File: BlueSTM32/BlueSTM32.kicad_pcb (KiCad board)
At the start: 4 copper layers, 40 x 40 mm, 63 parts, among them J1 TC2030-NL, J2 522071233, J3 USB4500-03-1-A_REVA, U1 OPA340NA, U2 BQ24040DSQR, U4 REF2033, U5 LT1304CS8-3.3-PBF, U6 LSM6DSRTR, U7 W25N02KVZEIR TR, U8 STM32WB55RGVx, X3 32.768kHz, X4 32MHz

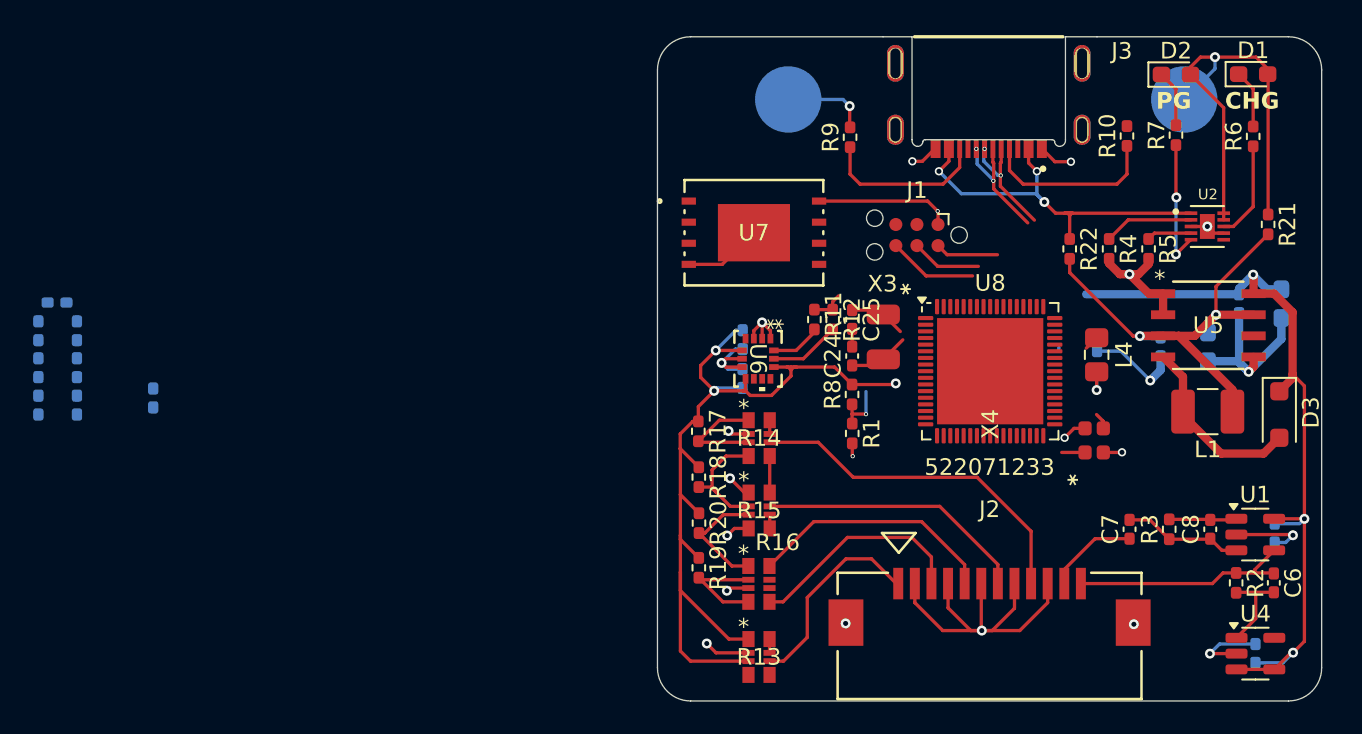
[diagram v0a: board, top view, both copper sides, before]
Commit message: Final layout of board
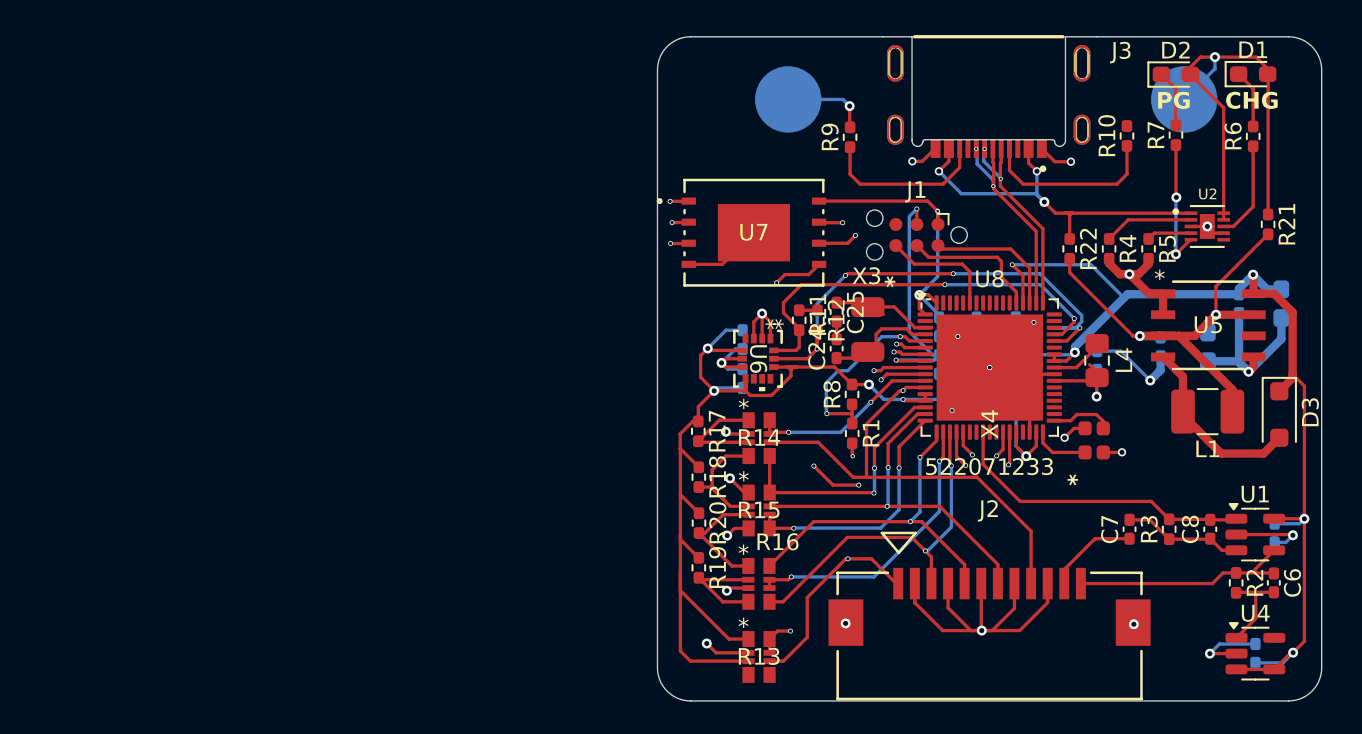
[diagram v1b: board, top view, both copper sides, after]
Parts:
- moved C18 58.9 mm to (171.6, 117.5), turned to 90 degrees
- moved C16 56.6 mm to (171.6, 119.7)
- moved C19 55.5 mm to (169.2, 119.7), turned to -90 degrees
- moved C20 54.4 mm to (167.0, 117.5)
- moved C21 54.4 mm to (169.2, 117.5), turned to -90 degrees
- moved C17 54.3 mm to (169.2, 122.0), turned to -90 degrees
- moved C1 54.2 mm to (167.0, 119.7), turned to -90 degrees
- moved C22 52.0 mm to (171.6, 122.0), turned to 90 degrees
- moved C25 1.03 mm to (160.8, 116.6)
- moved C24 1.03 mm to (160.8, 118.8)
- moved X3 1.03 mm to (162.7, 116.3)
- moved R12 0.92 mm to (159.6, 117.1)
- moved R11 0.92 mm to (158.5, 117.1)
- moved L4 0.35 mm to (176.5, 119.5)
- moved U8 0.22 mm to (170.0, 119.9)
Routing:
- net +3V3: track 116.4 -> 170.8 mm, vias 7 -> 12
- net /Microcontroller/Flash_CS: track 0.00 -> 35.5 mm, vias 0 -> 2
- net /Microcontroller/Flash_WP(IO2): track 0.00 -> 31.7 mm, vias 0 -> 4
- net IMU_SCL: track 4.27 -> 30.5 mm, vias 0 -> 4
- net Thermistor_Sense_+: track 0.83 -> 23.4 mm, vias 0 -> 2
- net IMU_SDA: track 3.06 -> 25.3 mm, vias 0 -> 2
- net /Microcontroller/Flash_CLK: track 0.00 -> 22.1 mm, vias 0 -> 2
- net /Microcontroller/Flash_HOLD(IO3): track 0.00 -> 21.4 mm, vias 0 -> 2
- net GND: track 94.1 -> 114.0 mm, vias 22 -> 27
- net /Microcontroller/Flash_DO(IO1): track 0.00 -> 19.4 mm, vias 0 -> 2
- net Strain_4_Sense_+: track 0.00 -> 17.3 mm, vias 0 -> 2
- net /Microcontroller/SWD_RST: track 0.00 -> 15.4 mm, vias 0 -> 2
- net Thermistor_Sense_-: track 12.3 -> 27.4 mm, vias 0 -> 2
- net Piezoelectric_Out: track 4.08 -> 18.6 mm
- net Strain_3_Sense_+: track 0.83 -> 15.1 mm, vias 0 -> 2
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
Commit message: Better Final Layout
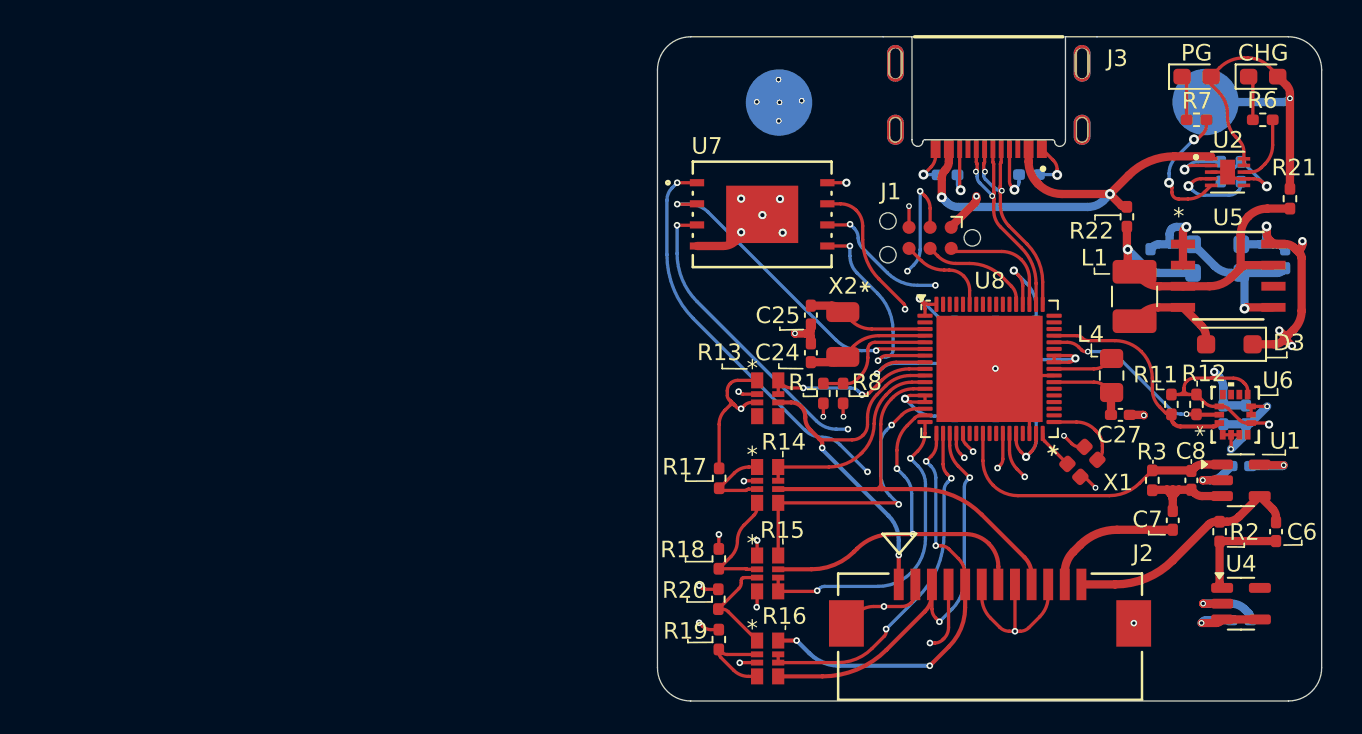
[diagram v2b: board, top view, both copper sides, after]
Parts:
- removed D1, D2: LED, LED_SMD:LED_0603_1608Metric_Pad1.05x0.95mm_HandSolder
- removed TP1: Battery_+, TestPoint:TestPoint_Pad_D4.0mm
- removed TP2: Battery_-, TestPoint:TestPoint_Pad_D4.0mm
- removed X3: 32.768kHz, Custom_Parts:32.768kHz Crystal
- added BAT+: Battery_+, TestPoint:TestPoint_Pad_D4.0mm, B.Cu at (183.0, 103.9)
- added CHG: LED, LED_SMD:LED_0603_1608Metric_Pad1.05x0.95mm_HandSolder, F.Cu at (186.5, 102.4)
- added GND: Battery_-, TestPoint:TestPoint_Pad_D4.0mm, B.Cu at (157.3, 104.0)
- added PG: LED, LED_SMD:LED_0603_1608Metric_Pad1.05x0.95mm_HandSolder, F.Cu at (182.5, 102.4)
- added X2: 32.768kHz, Custom_Parts:32.768kHz Crystal, F.Cu at (161.2, 116.6)
- C27: moved to F.Cu
- R10, R4, R5, R9: moved to B.Cu
- moved C10 30.6 mm to (185.4, 122.8)
- moved C11 29.0 mm to (184.1, 122.8), turned to -90 degrees
- moved U6 28.9 mm to (184.8, 122.8), turned to 90 degrees
- moved R12 23.4 mm to (182.5, 122.1)
- moved R11 23.0 mm to (180.9, 122.1)
- moved R13 15.6 mm to (156.6, 121.8)
- moved C12 11.3 mm to (185.1, 125.9), turned to 180 degrees
- moved L1 8.22 mm to (178.7, 115.6), turned to -90 degrees
- moved R4 8.18 mm to (183.9, 108.1)
- moved R5 7.25 mm to (185.1, 108.1), turned to 90 degrees
- moved R10 6.35 mm to (172.4, 108.3), turned to 0 degrees
- moved R9 6.29 mm to (167.5, 108.3), turned to 180 degrees
- moved C21 6.00 mm to (172.8, 122.3), turned to 90 degrees
- moved C20 5.90 mm to (170.4, 122.3), turned to 90 degrees
- moved C9 5.62 mm to (185.1, 135.1), turned to 0 degrees
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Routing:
- net +3V3: track 170.8 -> 98.8 mm, vias 12 -> 20
- net IMU_SCL: track 30.5 -> 11.6 mm, vias 4 -> 2
- net Thermistor_Sense_+: track 23.4 -> 10.5 mm
- net IMU_SDA: track 25.3 -> 13.4 mm, vias 2 -> 0
- net /Microcontroller/SWD_RST: track 15.4 -> 22.7 mm, vias 2 -> 3
- net Net-(J3-CC1): track 10.7 -> 3.56 mm, vias 0 -> 1
- net GND: track 114.0 -> 121.1 mm, vias 27 -> 35
- net Net-(J3-CC2): track 10.0 -> 3.49 mm, vias 0 -> 1
- net /Power/Reg_Vin: track 28.6 -> 22.5 mm, vias 2 -> 1
- net Net-(D3-A): track 11.2 -> 5.95 mm
- net /Power/USB_Vin: track 23.8 -> 28.5 mm, vias 3 -> 2
- net Strain_3_Sense_-: track 21.1 -> 25.7 mm, vias 2 -> 4
- net /Power/Battery_+: track 27.3 -> 23.0 mm
- net Thermistor_Sense_-: track 27.4 -> 23.1 mm
- net Strain_4_Sense_-: track 21.4 -> 25.5 mm
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- added copper zone on In2.Cu, net +3V3
- removed copper zone on In2.Cu, net GND
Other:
- board text added: "X1"
- board text removed: "${REFERENCE}"
- board text removed: "CHG"
- board text removed: "PG"
